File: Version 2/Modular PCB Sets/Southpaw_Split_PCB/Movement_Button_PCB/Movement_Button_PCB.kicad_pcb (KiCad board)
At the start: 2 copper layers, 111 x 115.6 mm, 13 parts, among them J6 Conn_01x06_Socket

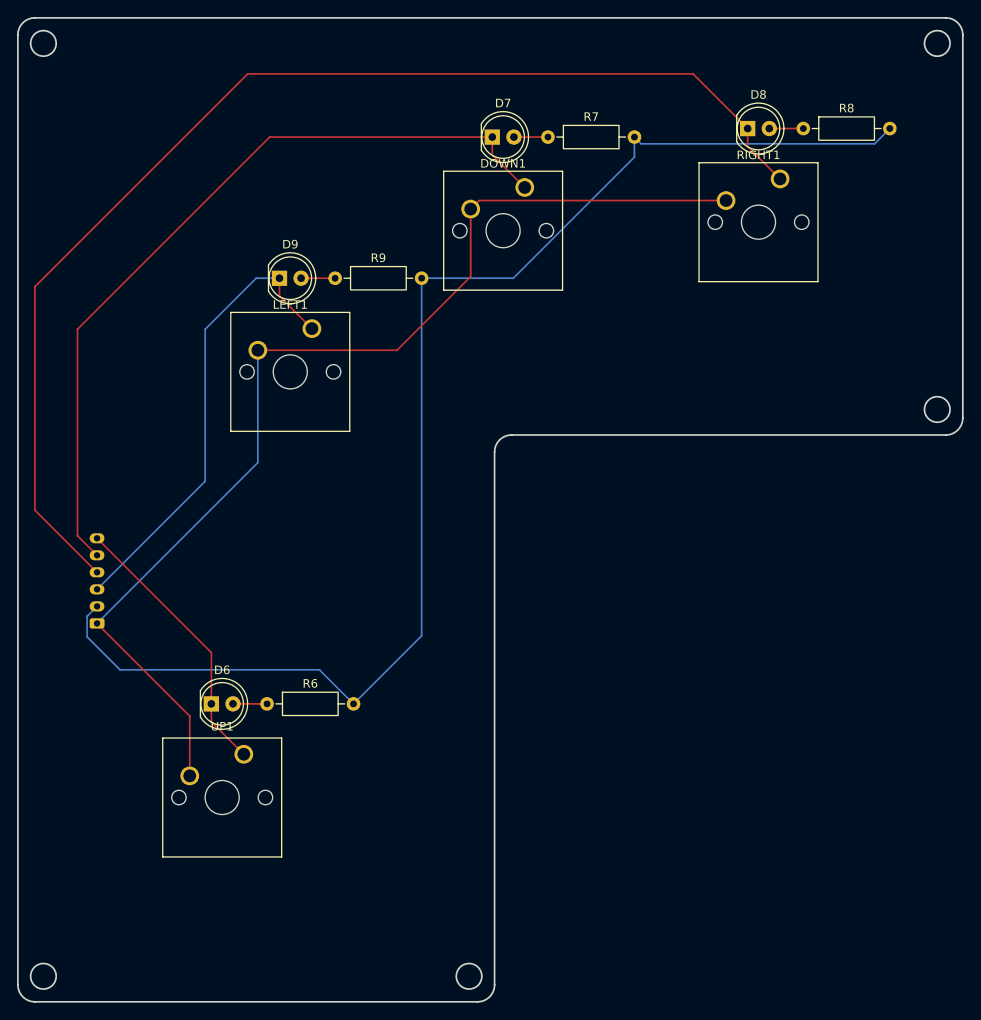
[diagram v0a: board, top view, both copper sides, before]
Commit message: Finalized design and uploaded gerbers to JLCpcb, waiting for boards to come in
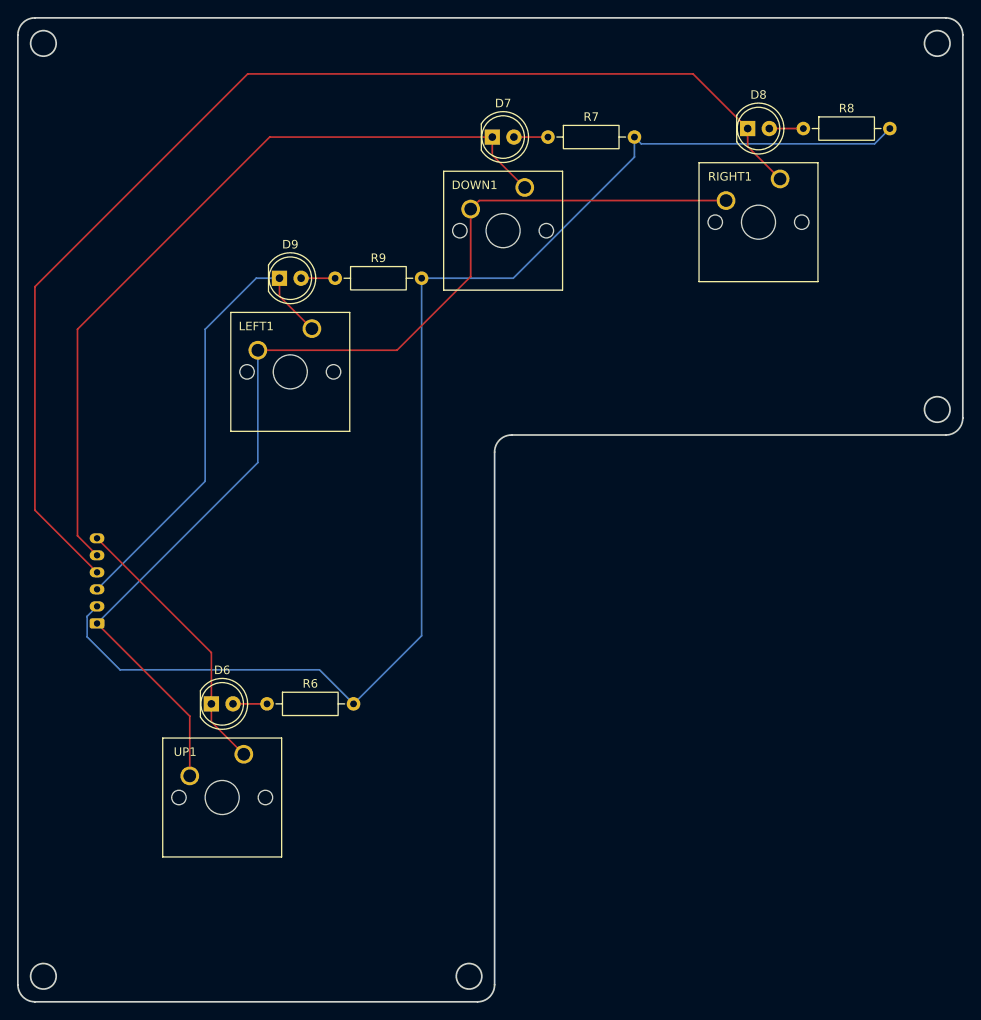
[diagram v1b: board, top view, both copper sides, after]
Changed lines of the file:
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@@
 			(plot_on_all_layers_selection 0x00000000_00000000_00000000_00000000)
 			(disableapertmacros no)
-			(usegerberextensions no)
+			(usegerberextensions yes)
 			(usegerberattributes yes)
 			(usegerberadvancedattributes yes)
-			(creategerberjobfile yes)
+			(creategerberjobfile no)
 			(dashed_line_dash_ratio 12.000000)
 			(dashed_line_gap_ratio 3.000000)
@@
 			(outputformat 1)
 			(mirror no)
-			(drillshape 1)
+			(drillshape 0)
 			(scaleselection 1)
-			(outputdirectory "")
+			(outputdirectory "../Gerbers/Movement_Button_Gerbers/")
 		)
 	)
@@
 		(tags "Cherry MX keyswitch 1.00u PCB")
 		(property "Reference" "DOWN1"
-			(at -2.54 -2.794 0)
+			(at -5.89 -0.27 0)
 			(layer "F.SilkS")
 			(effects
@@
 		)
 		(fp_text user "${REFERENCE}"
-			(at -2.54 -2.794 0)
+			(at -5.89 -0.27 0)
 			(layer "F.Fab")
 			(effects
@@
 		(tags "Cherry MX keyswitch 1.00u PCB")
 		(property "Reference" "LEFT1"
-			(at -2.54 -2.794 0)
+			(at -6.54 -0.27 0)
 			(layer "F.SilkS")
 			(effects
@@
 		)
 		(fp_text user "${REFERENCE}"
-			(at -2.54 -2.794 0)
+			(at -6.54 -0.27 0)
 			(layer "F.Fab")
 			(effects
@@
 		(tags "Cherry MX keyswitch 1.00u PCB")
 		(property "Reference" "UP1"
-			(at -2.54 -3.254 0)
+			(at -6.89 -0.27 0)
 			(layer "F.SilkS")
 			(effects
@@
 		)
 		(fp_text user "${REFERENCE}"
-			(at -2.54 -3.254 0)
+			(at -6.89 -0.27 0)
 			(layer "F.Fab")
 			(effects
@@
 		(tags "Cherry MX keyswitch 1.00u PCB")
 		(property "Reference" "RIGHT1"
-			(at -2.54 -2.794 0)
+			(at -5.89 -0.27 0)
 			(layer "F.SilkS")
 			(effects
@@
 		)
 		(fp_text user "${REFERENCE}"
-			(at -2.54 -2.794 0)
-			(layer "F.Fab")
-			(effects
+			(at -5.89 -0.27 0)
+			(layer "F.Fab")
+			(effects
